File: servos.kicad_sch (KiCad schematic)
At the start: 3 parts, among them J7 90120-0763, J8 90120-0763, J9 90120-0763

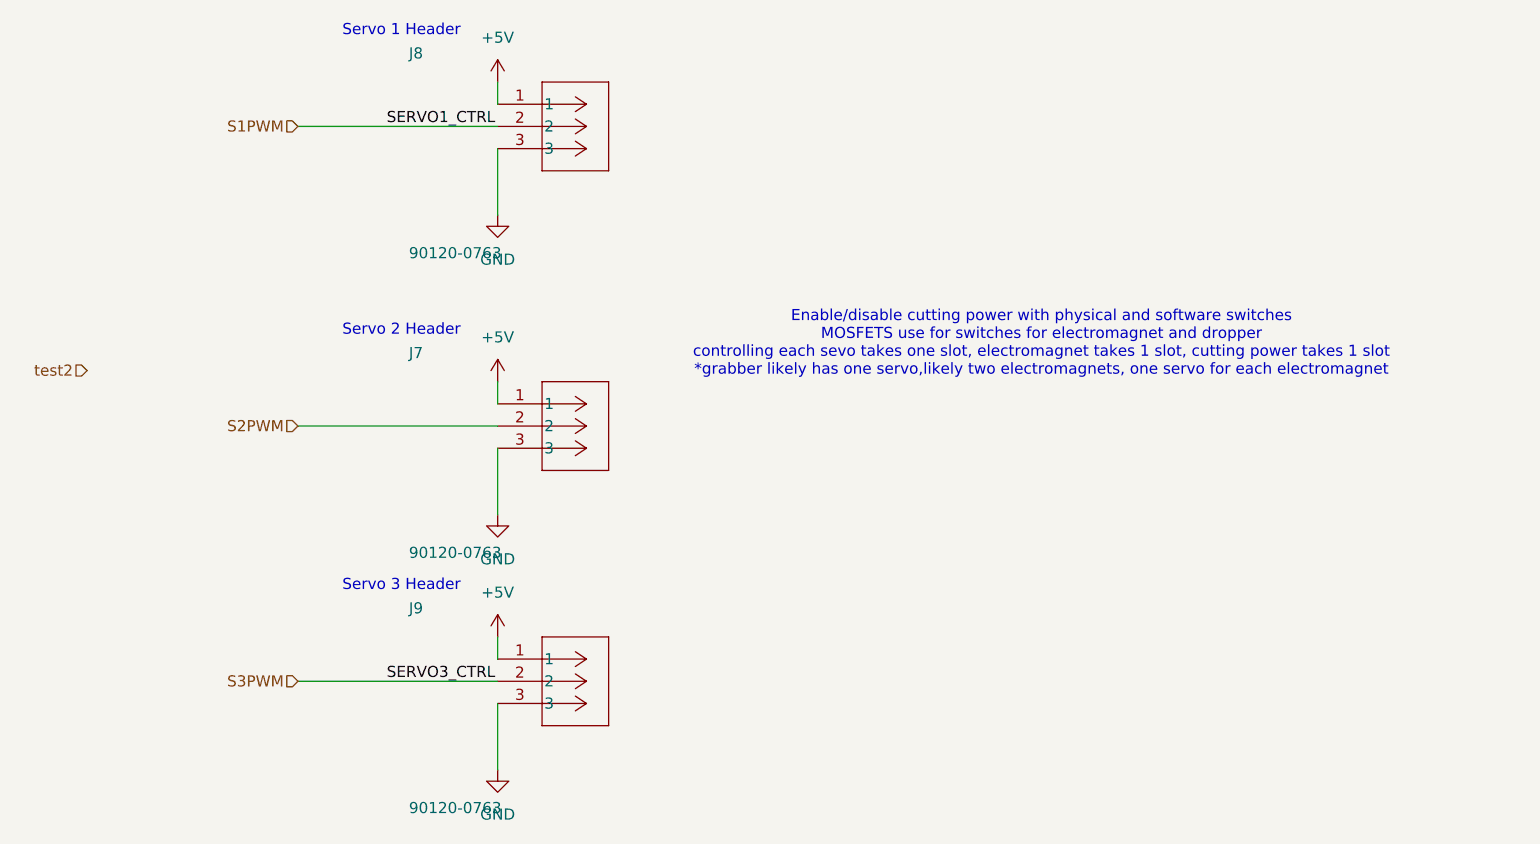
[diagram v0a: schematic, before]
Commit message: added footprints Servos on PCB
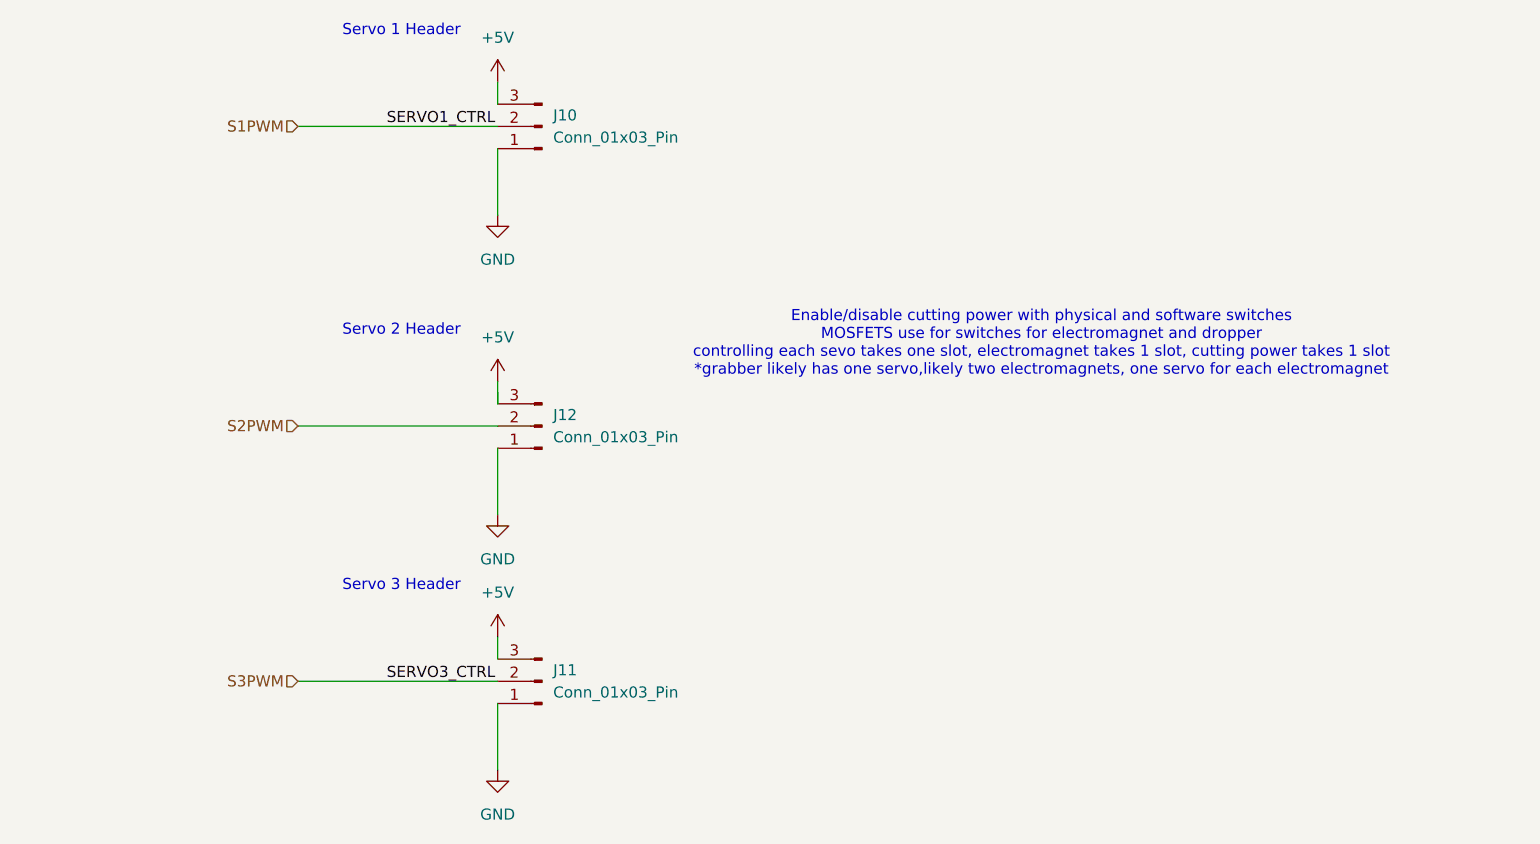
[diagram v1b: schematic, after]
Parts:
- removed J7, J8, J9: 90120-0763, CONN_901200763_MOL, symbol 2024-02-03_17-19-22:901200763
- added J10, J11, J12: Conn_01x03_Pin, Connector_PinHeader_2.54mm:PinHeader_1x03_P2.54mm_Vertical, symbol Connector:Conn_01x03_Pin
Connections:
- net +5V: now also J10.3 (Pin_3), J11.3 (Pin_3), J12.3 (Pin_3)
- net GND: now also J10.1 (Pin_1), J11.1 (Pin_1), J12.1 (Pin_1)
- net S1PWM: now also J10.2 (Pin_2)
- net S2PWM: now also J12.2 (Pin_2)
- net S3PWM: now also J11.2 (Pin_2)
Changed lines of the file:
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@@
 	(wire
 		(pts
-			(xy 97.79 88.9) (xy 97.79 86.36)
+			(xy 97.79 86.36) (xy 97.79 88.9)
 		)
 		(stroke
@@
 		(stroke
 			(width 0.254)
+			(type default)
+		)
+	)
+	(wire
+		(pts
+			(xy 97.79 88.9) (xy 97.79 87.63)
+		)
+		(stroke
+			(width 0)
 			(type default)
 		)
@@
 		)
 	)
-	(hierarchical_label "test2"
-		(shape input)
-		(at 50.8 85.09 180)
-		(effects
-			(font
-				(size 1.27 1.27)
-			)
-			(justify right)
-		)
-	)
-	(symbol
-		(lib_id "2024-02-03_17-19-22:901200763")
-		(at 97.79 118.11 0)
-		(unit 1)
-		(exclude_from_sim no)
-		(in_bom yes)
-		(on_board yes)
-		(dnp no)
-		(property "Reference" "J9"
-			(at 87.63 113.03 0)
-			(effects
-				(font
-					(size 1.27 1.27)
-				)
-				(justify left bottom)
-			)
-		)
-		(property "Value" "90120-0763"
-			(at 87.63 135.89 0)
-			(effects
-				(font
-					(size 1.27 1.27)
-				)
-				(justify left bottom)
-			)
-		)
-		(property "Footprint" "CONN_901200763_MOL"
-			(at 97.79 118.11 0)
-			(effects
-				(font
-					(size 1.27 1.27)
-					(italic yes)
-				)
-				(hide yes)
-			)
-		)
-		(property "Datasheet" "901200763"
-			(at 97.79 118.11 0)
-			(effects
-				(font
-					(size 1.27 1.27)
-					(italic yes)
-				)
-				(hide yes)
-			)
-		)
-		(property "Description" ""
-			(at 97.79 118.11 0)
-			(effects
-				(font
-					(size 1.27 1.27)
-				)
-			)
-		)
-		(property "Part Number" "90120-0763"
-			(at 97.79 118.11 0)
-			(effects
-				(font
-					(size 1.27 1.27)
-				)
-				(hide yes)
-			)
-		)
-		(pin "1"
+	(symbol
+		(lib_id "Connector:Conn_01x03_Pin")
+		(at 102.87 120.65 180)
+		(unit 1)
+		(exclude_from_sim no)
+		(in_bom yes)
+		(on_board yes)
+		(dnp no)
+		(fields_autoplaced yes)
+		(property "Reference" "J11"
+			(at 104.14 119.3799 0)
+			(effects
+				(font
+					(size 1.27 1.27)
+				)
+				(justify right)
+			)
+		)
+		(property "Value" "Conn_01x03_Pin"
+			(at 104.14 121.9199 0)
+			(effects
+				(font
+					(size 1.27 1.27)
+				)
+				(justify right)
+			)
+		)
+		(property "Footprint" "Connector_PinHeader_2.54mm:PinHeader_1x03_P2.54mm_Vertical"
+			(at 102.87 120.65 0)
+			(effects
+				(font
+					(size 1.27 1.27)
+				)
+				(hide yes)
+			)
+		)
+		(property "Datasheet" "~"
+			(at 102.87 120.65 0)
+			(effects
+				(font
+					(size 1.27 1.27)
+				)
+				(hide yes)
+			)
+		)
+		(property "Description" "Generic connector, single row, 01x03, script generated"
+			(at 102.87 120.65 0)
+			(effects
+				(font
+					(size 1.27 1.27)
+				)
+				(hide yes)
+			)
+		)
+		(pin "1"
+		)
+		(pin "3"
 		)
 		(pin "2"
 		)
-		(pin "3"
-		)
 		(instances
 			(project "Expansion_dual_header"
 				(path "/45910b0a-2ab6-4912-b705-1582171f57d5/5f2248db-3d7b-40c1-9259-f6fc27549d5d"
-					(reference "J9")
+					(reference "J11")
 					(unit 1)
 				)
@@
 	)
 	(symbol
-		(lib_id "2024-02-03_17-19-22:901200763")
-		(at 97.79 88.9 0)
-		(unit 1)
-		(exclude_from_sim no)
-		(in_bom yes)
-		(on_board yes)
-		(dnp no)
-		(property "Reference" "J7"
-			(at 87.63 83.82 0)
-			(effects
-				(font
-					(size 1.27 1.27)
-				)
-				(justify left bottom)
-			)
-		)
-		(property "Value" "90120-0763"
-			(at 87.63 106.68 0)
-			(effects
-				(font
-					(size 1.27 1.27)
-				)
-				(justify left bottom)
-			)
-		)
-		(property "Footprint" "CONN_901200763_MOL"
-			(at 97.79 88.9 0)
-			(effects
-				(font
-					(size 1.27 1.27)
-					(italic yes)
-				)
-				(hide yes)
-			)
-		)
-		(property "Datasheet" "901200763"
-			(at 97.79 88.9 0)
-			(effects
-				(font
-					(size 1.27 1.27)
-					(italic yes)
-				)
-				(hide yes)
-			)
-		)
-		(property "Description" ""
-			(at 97.79 88.9 0)
-			(effects
-				(font
-					(size 1.27 1.27)
-				)
-			)
-		)
-		(property "Part Number" "90120-0763"
-			(at 97.79 88.9 0)
-			(effects
-				(font
-					(size 1.27 1.27)
-				)
-				(hide yes)
-			)
-		)
-		(pin "1"
-		)
-		(pin "2"
-		)
-		(pin "3"
-		)
-		(instances
-			(project "Expansion_dual_header"
-				(path "/45910b0a-2ab6-4912-b705-1582171f57d5/5f2248db-3d7b-40c1-9259-f6fc27549d5d"
-					(reference "J7")
-					(unit 1)
-				)
-			)
-		)
-	)
-	(symbol
 		(lib_id "power:GND")
 		(at 97.79 67.31 0)
@@
 	)
 	(symbol
-		(lib_id "2024-02-03_17-19-22:901200763")
-		(at 97.79 54.61 0)
-		(unit 1)
-		(exclude_from_sim no)
-		(in_bom yes)
-		(on_board yes)
-		(dnp no)
-		(property "Reference" "J8"
-			(at 87.63 49.53 0)
-			(effects
-				(font
-					(size 1.27 1.27)
-				)
-				(justify left bottom)
-			)
-		)
-		(property "Value" "90120-0763"
-			(at 87.63 72.39 0)
-			(effects
-				(font
-					(size 1.27 1.27)
-				)
-				(justify left bottom)
-			)
-		)
-		(property "Footprint" "CONN_901200763_MOL"
-			(at 97.79 54.61 0)
-			(effects
-				(font
-					(size 1.27 1.27)
-					(italic yes)
-				)
-				(hide yes)
-			)
-		)
-		(property "Datasheet" "901200763"
-			(at 97.79 54.61 0)
-			(effects
-				(font
-					(size 1.27 1.27)
-					(italic yes)
-				)
-				(hide yes)
-			)
-		)
-		(property "Description" ""
-			(at 97.79 54.61 0)
-			(effects
-				(font
-					(size 1.27 1.27)
-				)
-			)
-		)
-		(property "Part Number" "90120-0763"
-			(at 97.79 54.61 0)
-			(effects
-				(font
-					(size 1.27 1.27)
-				)
-				(hide yes)
-			)
-		)
-		(pin "1"
+		(lib_id "Connector:Conn_01x03_Pin")
+		(at 102.87 57.15 180)
+		(unit 1)
+		(exclude_from_sim no)
+		(in_bom yes)
+		(on_board yes)
+		(dnp no)
+		(fields_autoplaced yes)
+		(property "Reference" "J10"
+			(at 104.14 55.8799 0)
+			(effects
+				(font
+					(size 1.27 1.27)
+				)
+				(justify right)
+			)
+		)
+		(property "Value" "Conn_01x03_Pin"
+			(at 104.14 58.4199 0)
+			(effects
+				(font
+					(size 1.27 1.27)
+				)
+				(justify right)
+			)
+		)
+		(property "Footprint" "Connector_PinHeader_2.54mm:PinHeader_1x03_P2.54mm_Vertical"
+			(at 102.87 57.15 0)
+			(effects
+				(font
+					(size 1.27 1.27)
+				)
+				(hide yes)
+			)
+		)
+		(property "Datasheet" "~"
+			(at 102.87 57.15 0)
+			(effects
+				(font
+					(size 1.27 1.27)
+				)
+				(hide yes)
+			)
+		)
+		(property "Description" "Generic connector, single row, 01x03, script generated"
+			(at 102.87 57.15 0)
+			(effects
+				(font
+					(size 1.27 1.27)
+				)
+				(hide yes)
+			)
+		)
+		(pin "1"
+		)
+		(pin "3"
 		)
 		(pin "2"
 		)
+		(instances
+			(project ""
+				(path "/45910b0a-2ab6-4912-b705-1582171f57d5/5f2248db-3d7b-40c1-9259-f6fc27549d5d"
+					(reference "J10")
+					(unit 1)
+				)
+			)
+		)
+	)
+	(symbol
+		(lib_id "Connector:Conn_01x03_Pin")
+		(at 102.87 91.44 180)
+		(unit 1)
+		(exclude_from_sim no)
+		(in_bom yes)
+		(on_board yes)
+		(dnp no)
+		(fields_autoplaced yes)
+		(property "Reference" "J12"
+			(at 104.14 90.1699 0)
+			(effects
+				(font
+					(size 1.27 1.27)
+				)
+				(justify right)
+			)
+		)
+		(property "Value" "Conn_01x03_Pin"
+			(at 104.14 92.7099 0)
+			(effects
+				(font
+					(size 1.27 1.27)
+				)
+				(justify right)
+			)
+		)
+		(property "Footprint" "Connector_PinHeader_2.54mm:PinHeader_1x03_P2.54mm_Vertical"
+			(at 102.87 91.44 0)
+			(effects
+				(font
+					(size 1.27 1.27)
+				)
+				(hide yes)
+			)
+		)
+		(property "Datasheet" "~"
+			(at 102.87 91.44 0)
+			(effects
+				(font
+					(size 1.27 1.27)
+				)
+				(hide yes)
+			)
+		)
+		(property "Description" "Generic connector, single row, 01x03, script generated"
+			(at 102.87 91.44 0)
+			(effects
+				(font
+					(size 1.27 1.27)
+				)
+				(hide yes)
+			)
+		)
+		(pin "1"
+		)
 		(pin "3"
 		)
+		(pin "2"
+		)
 		(instances
 			(project "Expansion_dual_header"
 				(path "/45910b0a-2ab6-4912-b705-1582171f57d5/5f2248db-3d7b-40c1-9259-f6fc27549d5d"
-					(reference "J8")
-					(unit 1)
-				)
+					(reference "J12")
+					(unit 1)
+				)
